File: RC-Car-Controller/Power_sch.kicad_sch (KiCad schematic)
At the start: 21 parts, among them J4 Conn_01x02_Pin, U2 A6986F3V3TR

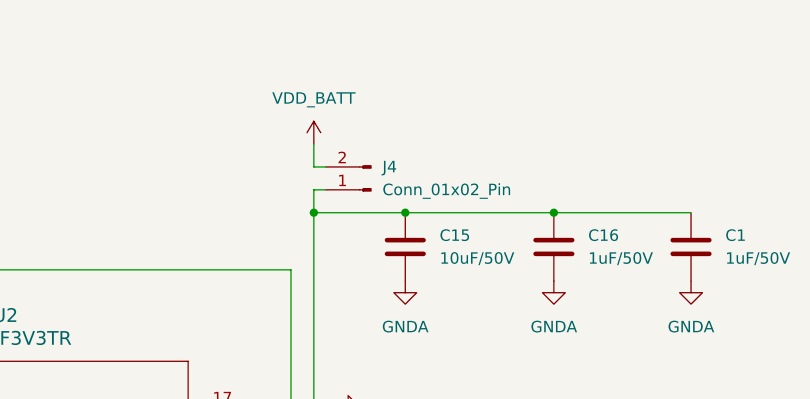
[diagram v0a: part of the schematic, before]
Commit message: Finished prelim. Controller
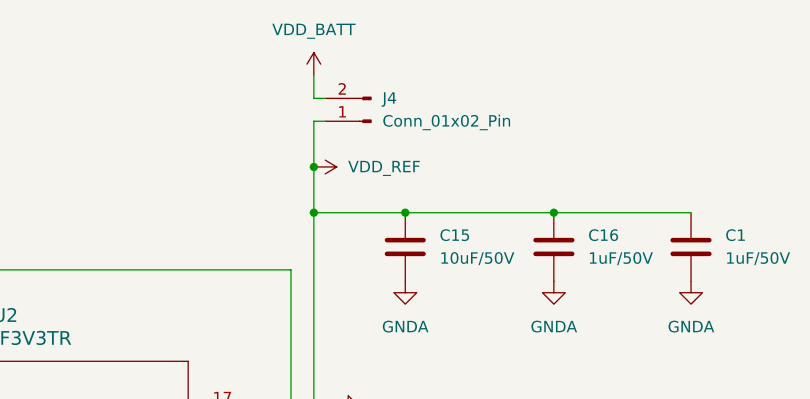
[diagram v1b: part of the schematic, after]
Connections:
- net VDD_REF: now reaches C1.1, C15.1, C16.1, J4.1 (Pin_1), U2.15 (VIN)
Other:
- moved on the sheet: J4
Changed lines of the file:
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@@
 	)
 	(junction
+		(at 176.53 73.66)
+		(diameter 0)
+		(color 0 0 0 0)
+	)
+	(junction
 		(at 170.18 107.95)
 		(diameter 0)
@@
 	(wire
 		(pts
+			(xy 176.53 73.66) (xy 176.53 78.74)
+		)
+		(stroke
+			(width 0)
+			(type default)
+		)
+	)
+	(wire
+		(pts
 			(xy 82.55 125.73) (xy 100.33 125.73)
 		)
@@
 	(wire
 		(pts
-			(xy 176.53 76.2) (xy 176.53 78.74)
+			(xy 176.53 68.58) (xy 176.53 73.66)
 		)
 		(stroke
@@
 	(wire
 		(pts
-			(xy 177.8 76.2) (xy 176.53 76.2)
+			(xy 177.8 68.58) (xy 176.53 68.58)
 		)
 		(stroke
@@
 	(wire
 		(pts
-			(xy 177.8 73.66) (xy 176.53 73.66)
+			(xy 177.8 66.04) (xy 176.53 66.04)
 		)
 		(stroke
@@
 	(wire
 		(pts
-			(xy 176.53 73.66) (xy 176.53 71.12)
+			(xy 176.53 66.04) (xy 176.53 63.5)
 		)
 		(stroke
@@
 	(symbol
 		(lib_id "power:+3V3")
-		(at 176.53 71.12 0)
+		(at 176.53 63.5 0)
 		(unit 1)
 		(exclude_from_sim no)
@@
 		(fields_autoplaced yes)
 		(property "Reference" "#PWR015"
-			(at 176.53 74.93 0)
+			(at 176.53 67.31 0)
 			(effects
 				(font
@@
 		)
 		(property "Value" "VDD_BATT"
-			(at 176.53 66.04 0)
+			(at 176.53 58.42 0)
 			(effects
 				(font
@@
 		)
 		(property "Footprint" ""
-			(at 176.53 71.12 0)
+			(at 176.53 63.5 0)
 			(effects
 				(font
@@
 		)
 		(property "Datasheet" ""
-			(at 176.53 71.12 0)
+			(at 176.53 63.5 0)
 			(effects
 				(font
@@
 		)
 		(property "Description" "Power symbol creates a global label with name \"+3V3\""
-			(at 176.53 71.12 0)
+			(at 176.53 63.5 0)
 			(effects
 				(font
@@
 	)
 	(symbol
+		(lib_id "power:+3V3")
+		(at 176.53 73.66 270)
+		(unit 1)
+		(exclude_from_sim no)
+		(in_bom yes)
+		(on_board yes)
+		(dnp no)
+		(fields_autoplaced yes)
+		(property "Reference" "#PWR033"
+			(at 172.72 73.66 0)
+			(effects
+				(font
+					(size 1.27 1.27)
+				)
+				(hide yes)
+			)
+		)
+		(property "Value" "VDD_REF"
+			(at 180.34 73.6599 90)
+			(effects
+				(font
+					(size 1.27 1.27)
+				)
+				(justify left)
+			)
+		)
+		(property "Footprint" ""
+			(at 176.53 73.66 0)
+			(effects
+				(font
+					(size 1.27 1.27)
+				)
+				(hide yes)
+			)
+		)
+		(property "Datasheet" ""
+			(at 176.53 73.66 0)
+			(effects
+				(font
+					(size 1.27 1.27)
+				)
+				(hide yes)
+			)
+		)
+		(property "Description" "Power symbol creates a global label with name \"+3V3\""
+			(at 176.53 73.66 0)
+			(effects
+				(font
+					(size 1.27 1.27)
+				)
+				(hide yes)
+			)
+		)
+		(pin "1"
+		)
+		(instances
+			(project "RC-Car-Controller"
+				(path "/ba870fd1-751d-4755-8e1a-1ea86ca9e2f6/e8cbdd69-5fc8-4583-a262-8a3c06e86dab"
+					(reference "#PWR033")
+					(unit 1)
+				)
+			)
+		)
+	)
+	(symbol
 		(lib_id "power:GND")
 		(at 227.33 118.11 0)
@@
 	(symbol
 		(lib_id "Connector:Conn_01x02_Pin")
-		(at 182.88 76.2 180)
+		(at 182.88 68.58 180)
 		(unit 1)
 		(exclude_from_sim no)
@@
 		(fields_autoplaced yes)
 		(property "Reference" "J4"
-			(at 184.15 73.6599 0)
+			(at 184.15 66.0399 0)
 			(effects
 				(font
@@
 		)
 		(property "Value" "Conn_01x02_Pin"
-			(at 184.15 76.1999 0)
+			(at 184.15 68.5799 0)
 			(effects
 				(font
@@
 		)
 		(property "Footprint" "Connector_PinHeader_2.54mm:PinHeader_1x02_P2.54mm_Vertical"
-			(at 182.88 76.2 0)
+			(at 182.88 68.58 0)
 			(effects
 				(font
@@
 		)
 		(property "Datasheet" "~"
-			(at 182.88 76.2 0)
+			(at 182.88 68.58 0)
 			(effects
 				(font
@@
 		)
 		(property "Description" "Generic connector, single row, 01x02, script generated"
-			(at 182.88 76.2 0)
+			(at 182.88 68.58 0)
 			(effects
 				(font

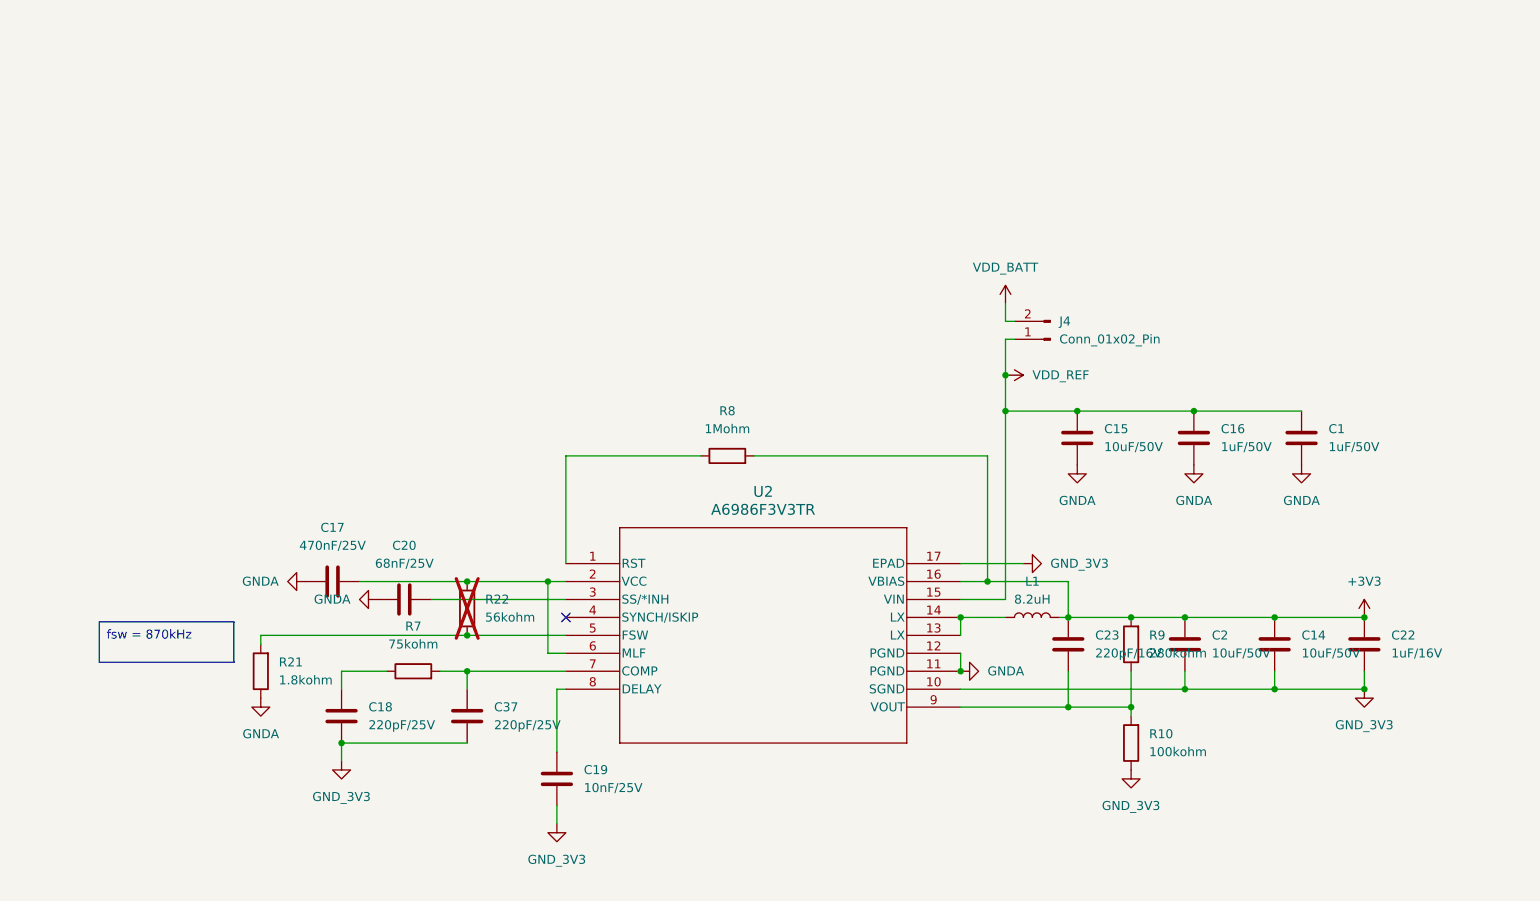
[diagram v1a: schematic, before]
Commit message: Did some stuff on the Controller
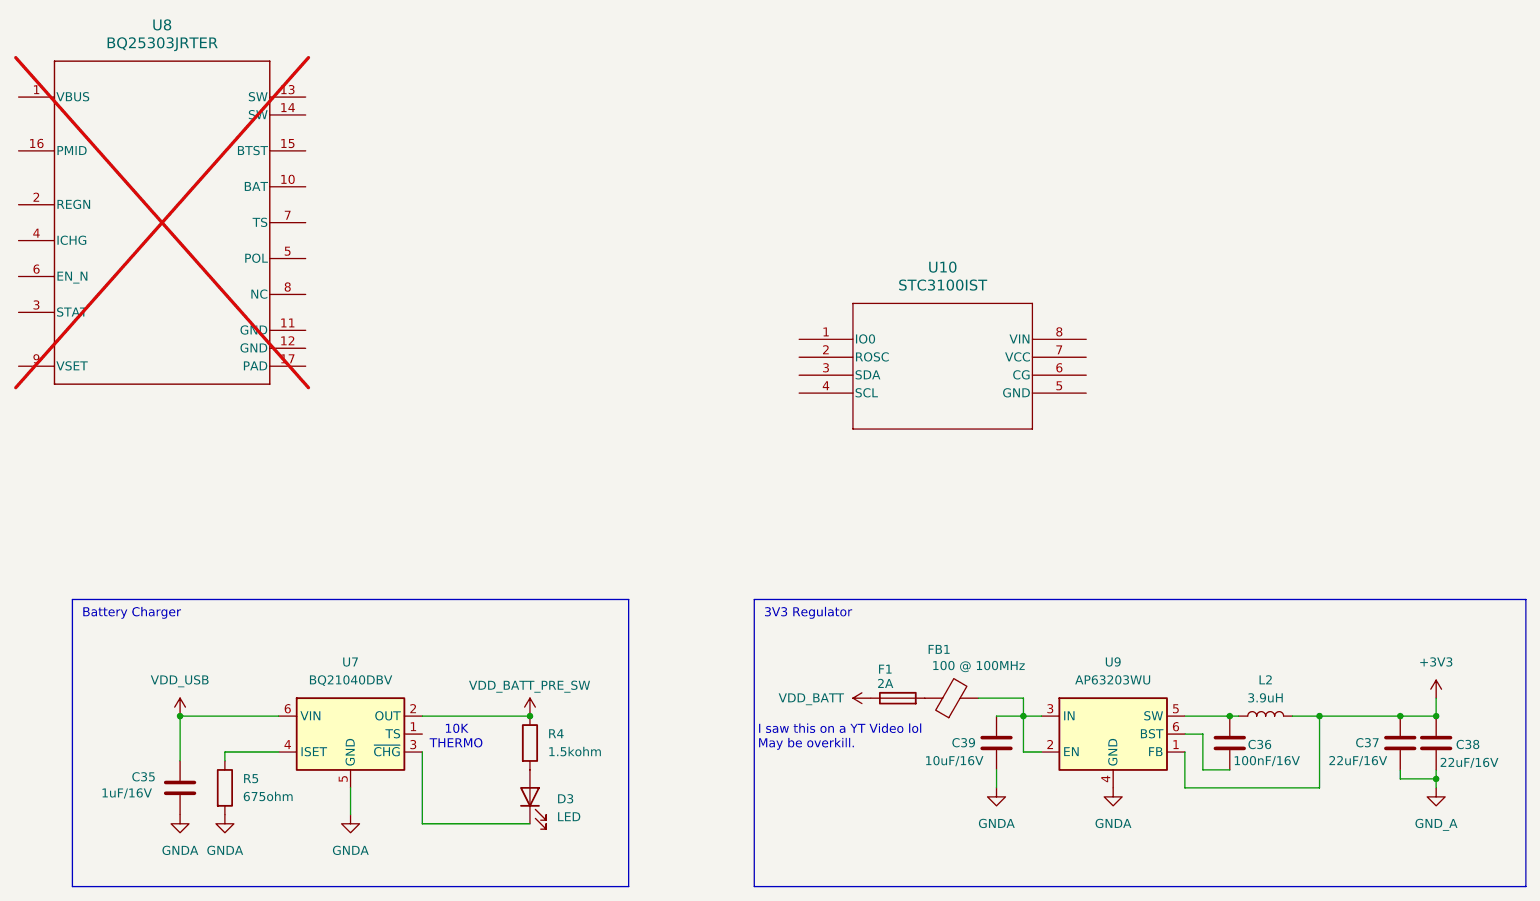
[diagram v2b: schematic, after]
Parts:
- removed C1, C16: 1uF/50V, Capacitor_SMD:C_0201_0603Metric, symbol Device:C
- removed C14, C15, C2: 10uF/50V, Capacitor_SMD:C_1210_3225Metric, symbol Device:C
- removed C17: 470nF/25V, Capacitor_SMD:C_0201_0603Metric, symbol Device:C
- removed C18: 220pF/25V, Capacitor_SMD:C_0201_0603Metric, symbol Device:C
- removed C19: 10nF/25V, Capacitor_SMD:C_0201_0603Metric, symbol Device:C
- removed C20: 68nF/25V, Capacitor_SMD:C_0201_0603Metric, symbol Device:C
- removed C22: 1uF/16V, Capacitor_SMD:C_0201_0603Metric, symbol Device:C
- removed C23: 220pF/16V, Capacitor_SMD:C_0201_0603Metric, symbol Device:C
- removed J4: Conn_01x02_Pin, Connector_PinHeader_2.54mm:PinHeader_1x02_P2.54mm_Vertical, symbol Connector:Conn_01x02_Pin
- removed L1: 8.2uH, Inductor_SMD:L_Wuerth_MAPI-4030, symbol Device:L
- removed R10: 100kohm, Resistor_SMD:R_0201_0603Metric, symbol Device:R
- removed R21: 1.8kohm, Resistor_SMD:R_0201_0603Metric, symbol Device:R
- removed R22: 56kohm, Resistor_SMD:R_0201_0603Metric, symbol Device:R
- removed R7: 75kohm, Resistor_SMD:R_0201_0603Metric, symbol Device:R
- removed R8: 1Mohm, Resistor_SMD:R_0201_0603Metric, symbol Device:R
- removed R9: 280kohm, Resistor_SMD:R_0201_0603Metric, symbol Device:R
- removed U2: A6986F3V3TR, footprints:HTSSOP16_4P5X5P1X0P65P_STM, symbol A6986F3V3TR:A6986F3V3TR
- added C35: 1uF/16V, Capacitor_SMD:C_0603_1608Metric, symbol Device:C
- added C36: 100nF/16V, Capacitor_SMD:C_0603_1608Metric, symbol Device:C
- added C38: 22uF/16V, Capacitor_SMD:C_0603_1608Metric, symbol Device:C
- added C39: 10uF/16V, Capacitor_SMD:C_0603_1608Metric, symbol Device:C
- added D3: LED, LED_SMD:LED_0603_1608Metric, symbol Device:LED
- added F1: 2A, symbol Device:Fuse
- added FB1: 100 @ 100MHz, symbol Device:FerriteBead
- added L2: 3.9uH, Inductor_SMD:L_Wuerth_MAPI-4030, symbol Device:L
- added R4: 1.5kohm, Resistor_SMD:R_0603_1608Metric, symbol Device:R
- added R5: 675ohm, Resistor_SMD:R_0603_1608Metric, symbol Device:R
- added U10: STC3100IST, MiniSO8_STM, symbol STC3100IST:STC3100IST
- added U7: BQ21040DBV, Package_TO_SOT_SMD:SOT-23-6, symbol Battery_Management:BQ21040DBV
- added U8: BQ25303JRTER, BQ25303JRTER:RTE0016C, symbol BQ25303JRTER:BQ25303JRTER
- added U9: AP63203WU, Package_TO_SOT_SMD:TSOT-23-6, symbol Regulator_Switching:AP63203WU
- C37: value 220pF/25V -> 22uF/16V; footprint Capacitor_SMD:C_0201_0603Metric -> Capacitor_SMD:C_0603_1608Metric
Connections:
- net GND_3V3 is gone; now on net +3V3: C37.1
- net +3V3: now also C38.1, L2.2, U9.1 (FB)
- net GNDA: now also C35.2, C39.2, R5.2, U7.5 (GND), U9.4 (GND)
- net VDD_BATT: now also F1.1
- net GND_A: now reaches C37.2
- net GND_A: now also C38.2
- new net: R5.1, U7.4 (ISET)
- new net: D3.1 (K), U7.3 (~{CHG})
- new net: D3.2 (A), R4.2
- new net: C39.1, FB1.2, U9.2 (EN), U9.3 (IN)
- new net: F1.2, FB1.1
- new net: C36.1, L2.1, U9.5 (SW)
- new net: C36.2, U9.6 (BST)
- new net VDD_BATT_PRE_SW: R4.1, U7.2 (OUT)
- new net VDD_USB: C35.1, U7.6 (VIN)
- no-connect marks 1 -> 0
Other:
- note added: "10K THERMO"
- note added: "3V3 Regulator"
- note added: "Battery Charger"
- note added: "I saw this on a YT Video lol May be overkill."
